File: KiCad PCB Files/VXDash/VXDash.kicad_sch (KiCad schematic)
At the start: 76 parts, among them IC1 CD74HC4050M96, J1 Header_VX220_RightAngle, J10 CANbus, J11 LD connector, J12 RD connector, J2 FASCIA PASSTHRU, J3 I²C debug, J4 UART0 debug, J5 CAN debug, SW1 RESET, SW2 BOOT, U1 TCA9555PWR, U2 ESP32-S3-WROOM-1

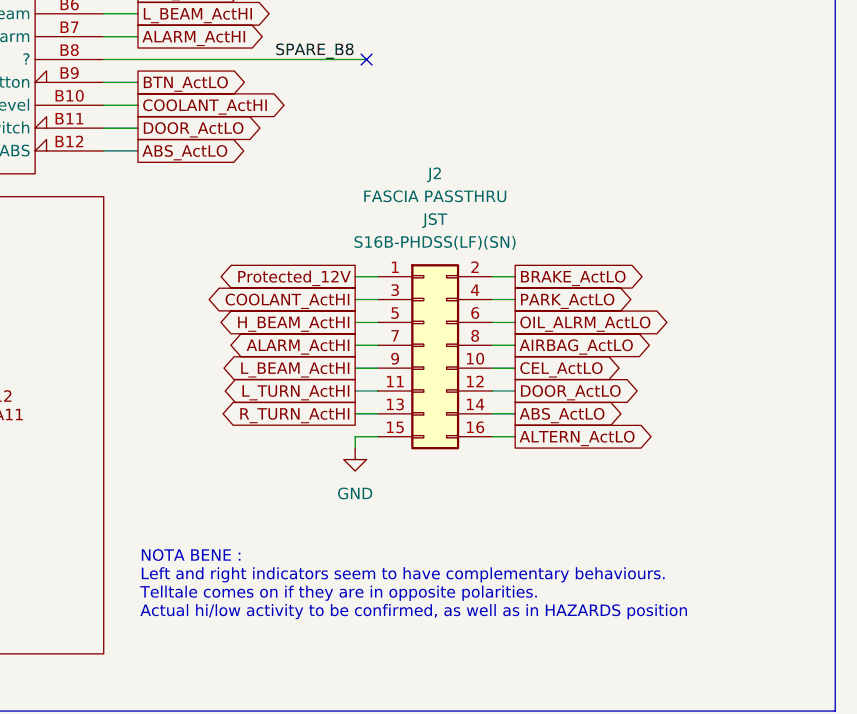
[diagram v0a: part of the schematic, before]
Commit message: Pre-grouping phase 2
It's tight yo
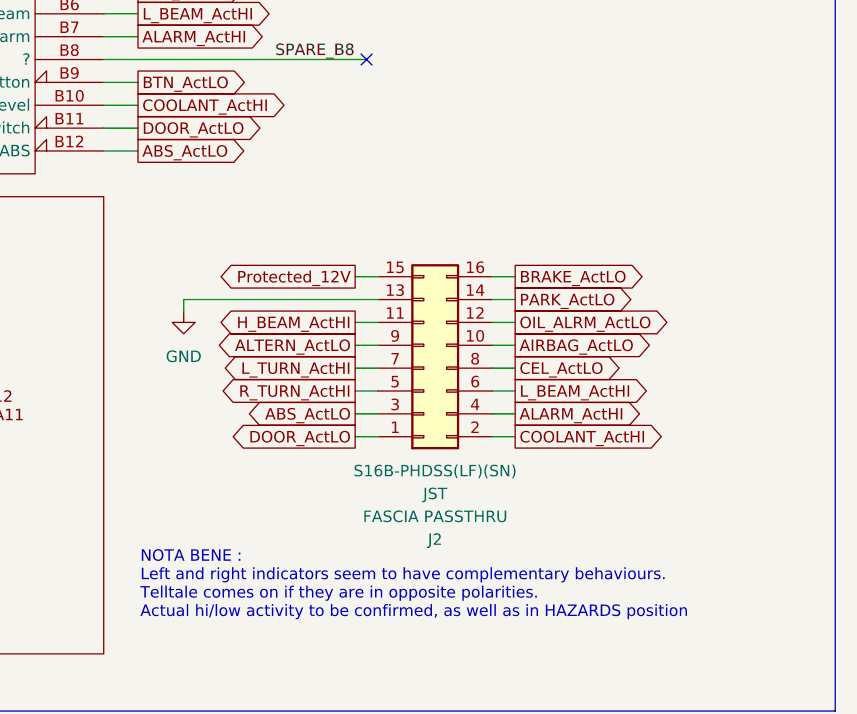
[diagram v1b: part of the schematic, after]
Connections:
- net ABS_ActLO: now also J2.3 (Pin_3); no longer J2.14 (Pin_14)
- net AIRBAG_ActLO: now also J2.10 (Pin_10); no longer J2.8 (Pin_8)
- net ALARM_ActHI: now also J2.4 (Pin_4); no longer J2.7 (Pin_7)
- net ALTERN_ActLO: now also J2.9 (Pin_9); no longer J2.16 (Pin_16)
- net BRAKE_ActLO: now also J2.16 (Pin_16); no longer J2.2 (Pin_2)
- net CEL_ActLO: now also J2.8 (Pin_8); no longer J2.10 (Pin_10)
- net COOLANT_ActHI: now also J2.2 (Pin_2); no longer J2.3 (Pin_3)
- net DOOR_ActLO: now also J2.1 (Pin_1); no longer J2.12 (Pin_12)
- net GND: now also J2.13 (Pin_13); no longer J2.15 (Pin_15)
- net H_BEAM_ActHI: now also J2.11 (Pin_11); no longer J2.5 (Pin_5)
- net L_BEAM_ActHI: now also J2.6 (Pin_6); no longer J2.9 (Pin_9)
- net L_TURN_ActHI: now also J2.7 (Pin_7); no longer J2.11 (Pin_11)
- net OIL_ALRM_ActLO: now also J2.12 (Pin_12); no longer J2.6 (Pin_6)
- net PARK_ActLO: now also J2.14 (Pin_14); no longer J2.4 (Pin_4)
- net Protected_12V: now also J2.15 (Pin_15); no longer J2.1 (Pin_1)
- net R_TURN_ActHI: now also J2.5 (Pin_5); no longer J2.13 (Pin_13)
